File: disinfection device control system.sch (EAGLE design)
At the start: 64 parts, among them J1 SENSOR JMP, J2 AVR_SPI, J3 SENSOR JMP, U1 MLX90614, U2 ATMEGA328P_TQFP, U3 SN74HC595N, U4 SN74HC595N

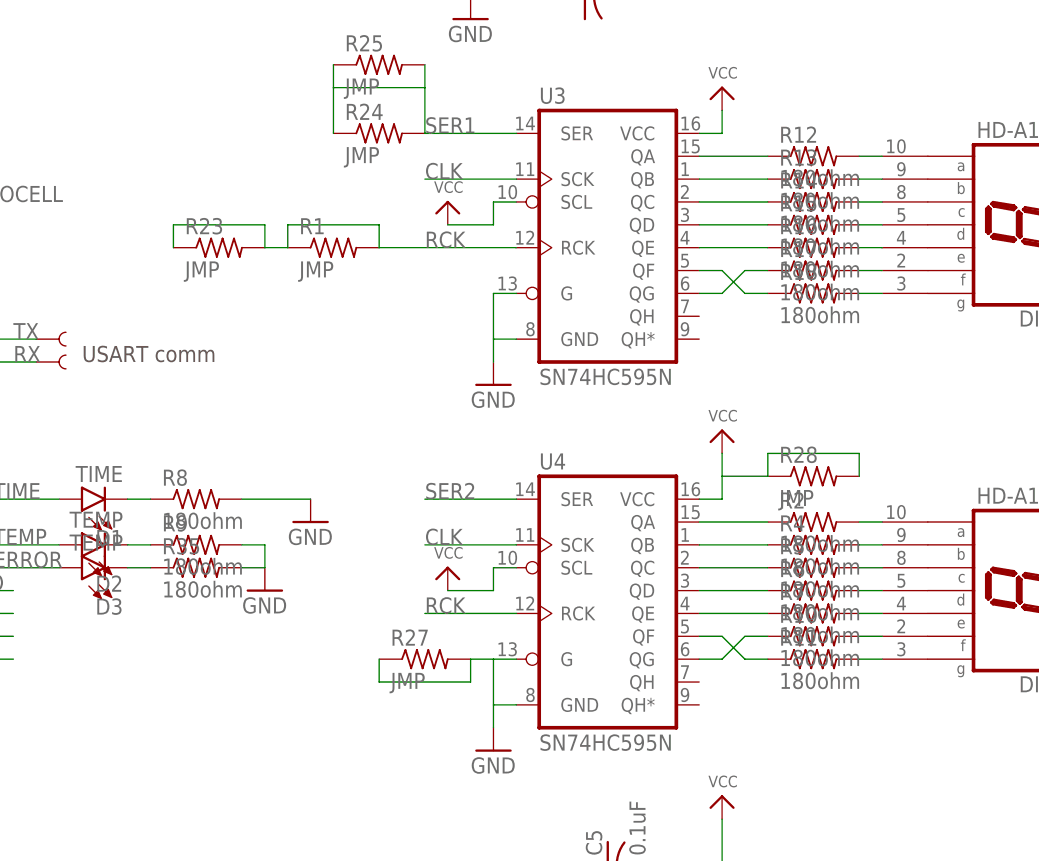
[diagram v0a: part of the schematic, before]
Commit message: Add files via upload
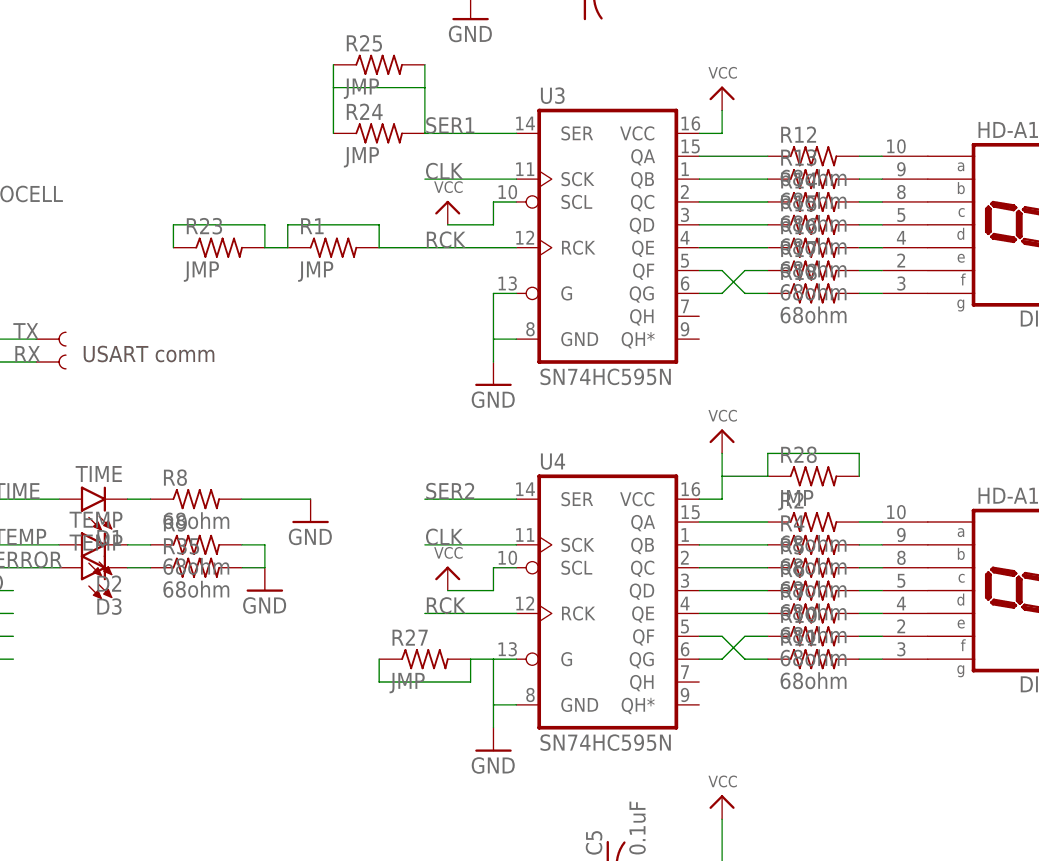
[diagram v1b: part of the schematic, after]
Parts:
- R10, R11, R12, R13, R14, R15, R16, R17, R18, R2, R35, R4, R5, R6, R7, R8, R9: value 180ohm -> 68ohm
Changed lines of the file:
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@@
 <part name="FRAME1" library="SparkFun-Retired" deviceset="FRAME-A3" device=""/>
 <part name="GND6" library="supply1" deviceset="GND" device=""/>
-<part name="R8" library="adafruit" deviceset="R-US_" device="R1206" value="180ohm"/>
-<part name="R9" library="adafruit" deviceset="R-US_" device="R1206" value="180ohm"/>
+<part name="R8" library="adafruit" deviceset="R-US_" device="R1206" value="68ohm"/>
+<part name="R9" library="adafruit" deviceset="R-US_" device="R1206" value="68ohm"/>
 <part name="DIS1" library="display-hp" deviceset="HD-A103" device=""/>
-<part name="R2" library="adafruit" deviceset="R-US_" device="R1206" value="180ohm"/>
-<part name="R4" library="adafruit" deviceset="R-US_" device="R1206" value="180ohm"/>
-<part name="R5" library="adafruit" deviceset="R-US_" device="R1206" value="180ohm"/>
-<part name="R6" library="adafruit" deviceset="R-US_" device="R1206" value="180ohm"/>
-<part name="R7" library="adafruit" deviceset="R-US_" device="R1206" value="180ohm"/>
-<part name="R10" library="adafruit" deviceset="R-US_" device="R1206" value="180ohm"/>
-<part name="R11" library="adafruit" deviceset="R-US_" device="R1206" value="180ohm"/>
+<part name="R2" library="adafruit" deviceset="R-US_" device="R1206" value="68ohm"/>
+<part name="R4" library="adafruit" deviceset="R-US_" device="R1206" value="68ohm"/>
+<part name="R5" library="adafruit" deviceset="R-US_" device="R1206" value="68ohm"/>
+<part name="R6" library="adafruit" deviceset="R-US_" device="R1206" value="68ohm"/>
+<part name="R7" library="adafruit" deviceset="R-US_" device="R1206" value="68ohm"/>
+<part name="R10" library="adafruit" deviceset="R-US_" device="R1206" value="68ohm"/>
+<part name="R11" library="adafruit" deviceset="R-US_" device="R1206" value="68ohm"/>
 <part name="GND7" library="supply1" deviceset="GND" device=""/>
 <part name="DIS2" library="display-hp" deviceset="HD-A103" device=""/>
-<part name="R12" library="adafruit" deviceset="R-US_" device="R1206" value="180ohm"/>
-<part name="R13" library="adafruit" deviceset="R-US_" device="R1206" value="180ohm"/>
-<part name="R14" library="adafruit" deviceset="R-US_" device="R1206" value="180ohm"/>
-<part name="R15" library="adafruit" deviceset="R-US_" device="R1206" value="180ohm"/>
-<part name="R16" library="adafruit" deviceset="R-US_" device="R1206" value="180ohm"/>
-<part name="R17" library="adafruit" deviceset="R-US_" device="R1206" value="180ohm"/>
-<part name="R18" library="adafruit" deviceset="R-US_" device="R1206" value="180ohm"/>
+<part name="R12" library="adafruit" deviceset="R-US_" device="R1206" value="68ohm"/>
+<part name="R13" library="adafruit" deviceset="R-US_" device="R1206" value="68ohm"/>
+<part name="R14" library="adafruit" deviceset="R-US_" device="R1206" value="68ohm"/>
+<part name="R15" library="adafruit" deviceset="R-US_" device="R1206" value="68ohm"/>
+<part name="R16" library="adafruit" deviceset="R-US_" device="R1206" value="68ohm"/>
+<part name="R17" library="adafruit" deviceset="R-US_" device="R1206" value="68ohm"/>
+<part name="R18" library="adafruit" deviceset="R-US_" device="R1206" value="68ohm"/>
 <part name="GND8" library="supply1" deviceset="GND" device=""/>
 <part name="D2" library="SparkFun-LED" deviceset="LED-RED" device="1206" value="TEMP"/>
@@
 <part name="R34" library="adafruit" deviceset="R-US_" device="R1206" value="JMP"/>
 <part name="D3" library="SparkFun-LED" deviceset="LED-RED" device="1206" value="TEMP"/>
-<part name="R35" library="adafruit" deviceset="R-US_" device="R1206" value="180ohm"/>
+<part name="R35" library="adafruit" deviceset="R-US_" device="R1206" value="68ohm"/>
 </parts>
 <sheets>
